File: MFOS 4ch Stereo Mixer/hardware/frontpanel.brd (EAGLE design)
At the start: 30.1 x 128.3 mm, 0 parts

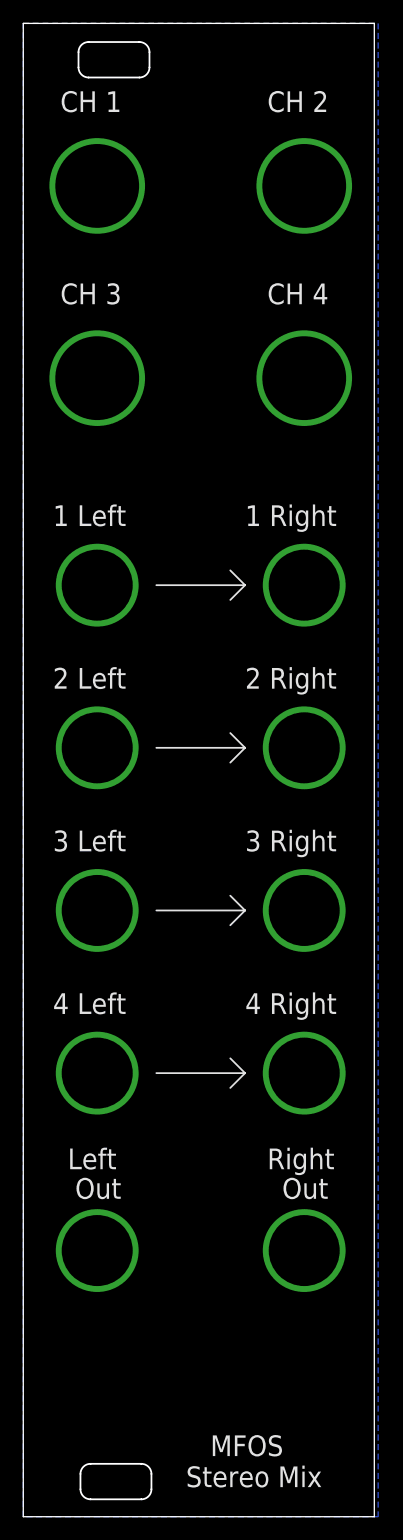
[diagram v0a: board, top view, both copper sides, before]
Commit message: Add files via upload
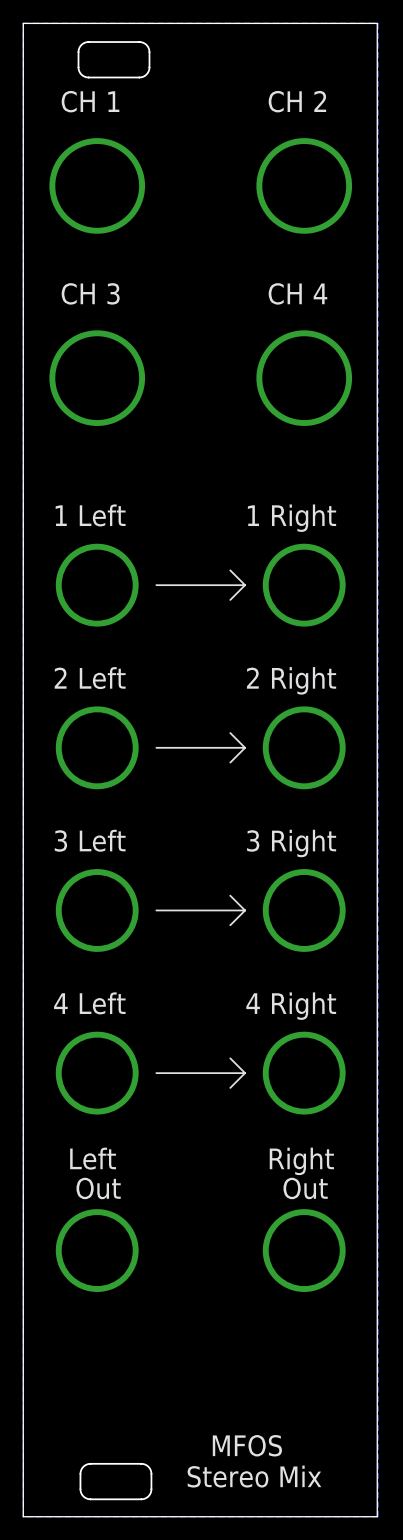
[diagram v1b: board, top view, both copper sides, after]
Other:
- board size 30.1 x 128.3 mm -> 30.4 x 128.3 mm
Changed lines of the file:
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@@
 <board>
 <plain>
-<wire x1="30.15" y1="128.26" x2="0" y2="128.26" width="0" layer="20"/>
+<wire x1="30.404" y1="128.26" x2="0" y2="128.26" width="0" layer="20"/>
 <wire x1="0" y1="128.26" x2="0" y2="0" width="0" layer="20"/>
-<wire x1="30.15" y1="0" x2="30.15" y2="128.26" width="0" layer="20"/>
-<wire x1="0" y1="0" x2="30.15" y2="0" width="0" layer="20"/>
+<wire x1="30.404" y1="0" x2="30.404" y2="128.26" width="0" layer="20"/>
+<wire x1="0" y1="0" x2="30.404" y2="0" width="0" layer="20"/>
 <text x="3.175" y="120.65" size="1.778" layer="25" font="vector">CH 1</text>
 <text x="20.955" y="120.65" size="1.778" layer="25" font="vector">CH 2</text>
